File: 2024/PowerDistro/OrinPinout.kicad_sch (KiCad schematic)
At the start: 5 parts, among them J19 4 Pin JST-GH, J20 4 Pin JST-GH, J21 4 Pin JST-GH, J22 4 Pin JST-GH

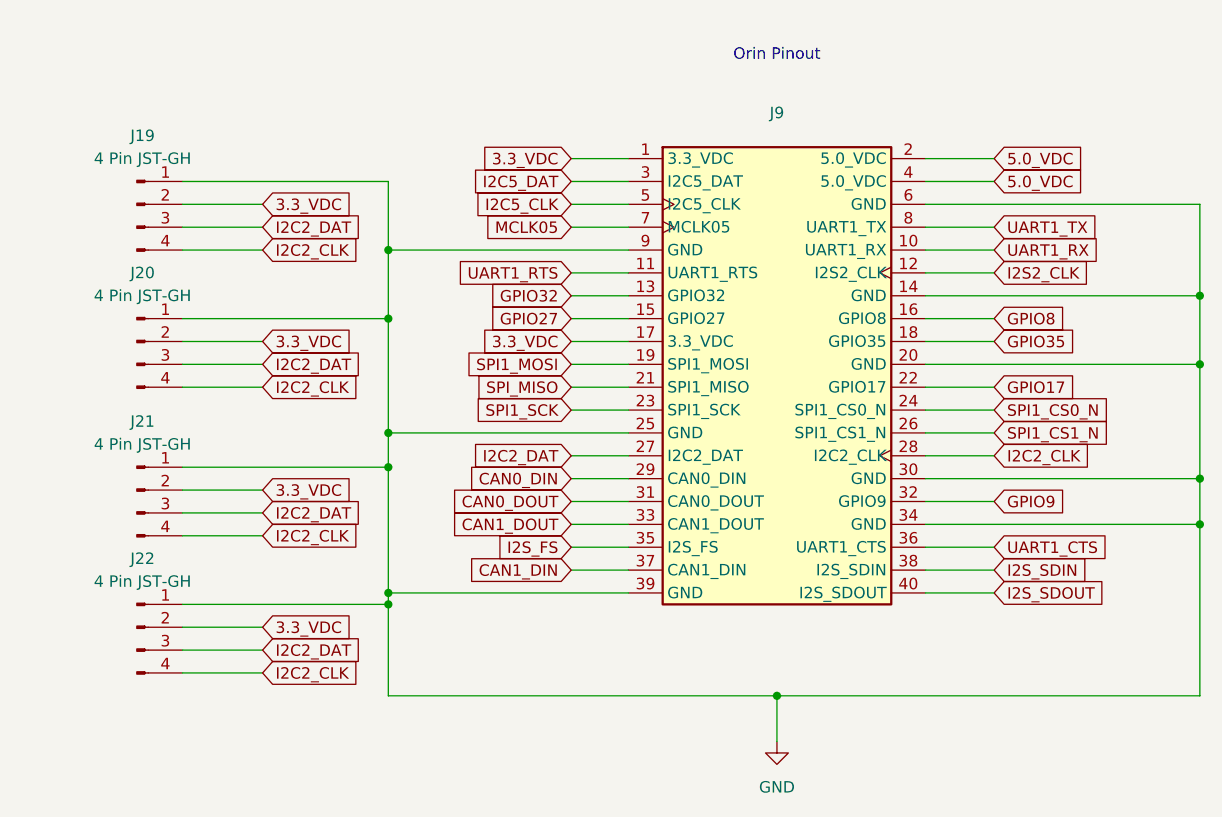
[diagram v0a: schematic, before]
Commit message: Changed Everything
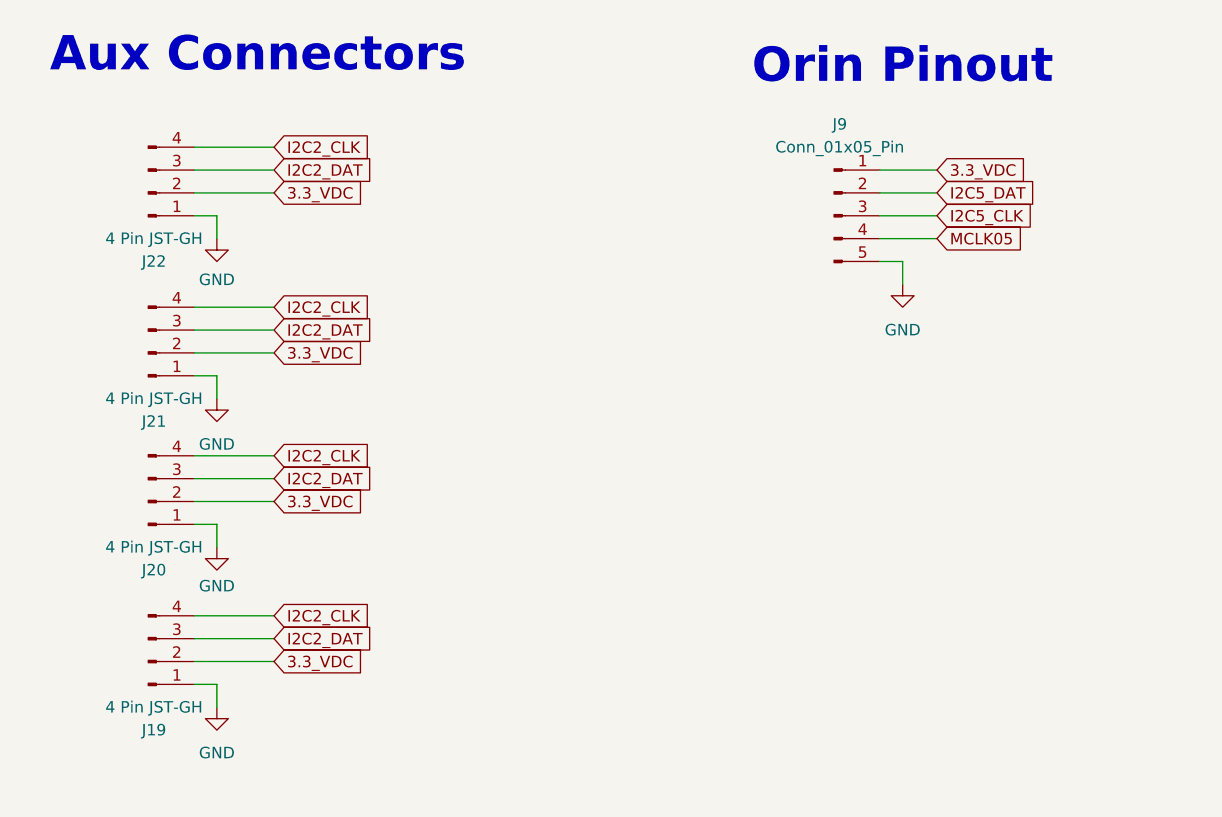
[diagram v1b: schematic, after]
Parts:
- removed J9: ~, Connector_PinHeader_2.54mm:PinHeader_2x20_P2.54mm_Vertical_SMD, symbol PowerDistro:JetsonAGXOrinExpansionHeader
- added J9: Conn_01x05_Pin, Connector_PinHeader_2.54mm:PinHeader_1x05_P2.54mm_Vertical, symbol Connector:Conn_01x05_Pin
- J19, J20, J21, J22: footprint PowerDistroFootprints:JST_BM04B-GHS-TBT_LF__SN__N_ -> Connector_JST:JST_XH_B4B-XH-A_1x04_P2.50mm_Vertical
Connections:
- net 3.3_VDC: now also J9.1 (Pin_1)
- net GND: now also J9.5 (Pin_5)
- net I2C5_CLK: now also J9.3 (Pin_3)
- net I2C5_DAT: now also J9.2 (Pin_2)
- net MCLK05: now also J9.4 (Pin_4)
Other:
- note added: "Aux Connectors"
- moved on the sheet: J19, J20, J21, J22

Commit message: Release
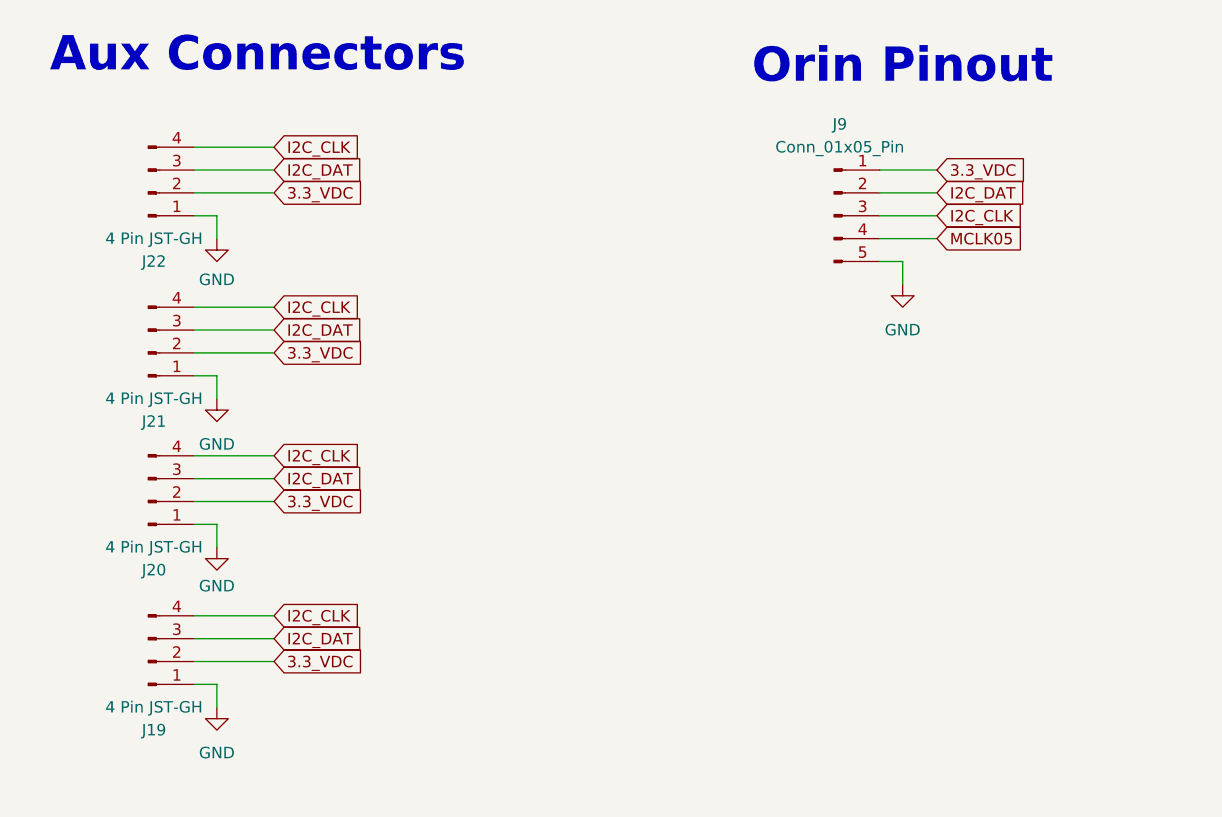
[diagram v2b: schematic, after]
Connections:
- net I2C5_CLK is gone; now on net I2C_CLK: J9.3 (Pin_3)
- net I2C5_DAT is gone; now on net I2C_DAT: J9.2 (Pin_2)
- net I2C2_CLK renamed I2C_CLK
- net I2C2_DAT renamed I2C_DAT
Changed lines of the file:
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@@
 		)
 	)
-	(global_label "I2C2_DAT"
+	(global_label "I2C_DAT"
 		(shape input)
 		(at 139.7 93.98 0)
@@
 		)
 		(property "Intersheetrefs" "${INTERSHEET_REFS}"
-			(at 151.2728 93.98 0)
+			(at 150.0633 93.98 0)
 			(effects
 				(font
@@
 		)
 	)
-	(global_label "I2C2_DAT"
+	(global_label "I2C_DAT"
 		(shape input)
 		(at 139.7 77.47 0)
@@
 		)
 		(property "Intersheetrefs" "${INTERSHEET_REFS}"
-			(at 151.2728 77.47 0)
-			(effects
-				(font
-					(size 1.27 1.27)
-				)
-				(justify left)
-				(hide yes)
-			)
-		)
-	)
-	(global_label "I2C2_CLK"
+			(at 150.0633 77.47 0)
+			(effects
+				(font
+					(size 1.27 1.27)
+				)
+				(justify left)
+				(hide yes)
+			)
+		)
+	)
+	(global_label "I2C_CLK"
 		(shape input)
 		(at 139.7 57.15 0)
@@
 		)
 		(property "Intersheetrefs" "${INTERSHEET_REFS}"
-			(at 151.5147 57.15 0)
-			(effects
-				(font
-					(size 1.27 1.27)
-				)
-				(justify left)
-				(hide yes)
-			)
-		)
-	)
-	(global_label "I2C2_CLK"
+			(at 150.3052 57.15 0)
+			(effects
+				(font
+					(size 1.27 1.27)
+				)
+				(justify left)
+				(hide yes)
+			)
+		)
+	)
+	(global_label "I2C_CLK"
 		(shape input)
 		(at 139.7 74.93 0)
@@
 		)
 		(property "Intersheetrefs" "${INTERSHEET_REFS}"
-			(at 151.5147 74.93 0)
+			(at 150.3052 74.93 0)
 			(effects
 				(font
@@
 		)
 	)
-	(global_label "I2C5_DAT"
+	(global_label "I2C_DAT"
 		(shape input)
 		(at 213.36 62.23 0)
@@
 		)
 		(property "Intersheetrefs" "${INTERSHEET_REFS}"
-			(at 224.9328 62.23 0)
+			(at 223.7233 62.23 0)
 			(effects
 				(font
@@
 		)
 	)
-	(global_label "I2C2_CLK"
+	(global_label "I2C_CLK"
 		(shape input)
 		(at 139.7 91.44 0)
@@
 		)
 		(property "Intersheetrefs" "${INTERSHEET_REFS}"
-			(at 151.5147 91.44 0)
-			(effects
-				(font
-					(size 1.27 1.27)
-				)
-				(justify left)
-				(hide yes)
-			)
-		)
-	)
-	(global_label "I2C2_DAT"
+			(at 150.3052 91.44 0)
+			(effects
+				(font
+					(size 1.27 1.27)
+				)
+				(justify left)
+				(hide yes)
+			)
+		)
+	)
+	(global_label "I2C_DAT"
 		(shape input)
 		(at 139.7 59.69 0)
@@
 		)
 		(property "Intersheetrefs" "${INTERSHEET_REFS}"
-			(at 151.2728 59.69 0)
+			(at 150.0633 59.69 0)
 			(effects
 				(font
@@
 		)
 	)
-	(global_label "I2C2_CLK"
+	(global_label "I2C_CLK"
 		(shape input)
 		(at 139.7 109.22 0)
@@
 		)
 		(property "Intersheetrefs" "${INTERSHEET_REFS}"
-			(at 151.5147 109.22 0)
-			(effects
-				(font
-					(size 1.27 1.27)
-				)
-				(justify left)
-				(hide yes)
-			)
-		)
-	)
-	(global_label "I2C2_DAT"
+			(at 150.3052 109.22 0)
+			(effects
+				(font
+					(size 1.27 1.27)
+				)
+				(justify left)
+				(hide yes)
+			)
+		)
+	)
+	(global_label "I2C_DAT"
 		(shape input)
 		(at 139.7 111.76 0)
@@
 		)
 		(property "Intersheetrefs" "${INTERSHEET_REFS}"
-			(at 151.2728 111.76 0)
-			(effects
-				(font
-					(size 1.27 1.27)
-				)
-				(justify left)
-				(hide yes)
-			)
-		)
-	)
-	(global_label "I2C5_CLK"
+			(at 150.0633 111.76 0)
+			(effects
+				(font
+					(size 1.27 1.27)
+				)
+				(justify left)
+				(hide yes)
+			)
+		)
+	)
+	(global_label "I2C_CLK"
 		(shape input)
 		(at 213.36 64.77 0)
@@
 		)
 		(property "Intersheetrefs" "${INTERSHEET_REFS}"
-			(at 225.1747 64.77 0)
-			(effects
-				(font
+			(at 223.9652 64.77 0)
+			(effects
+				(font
